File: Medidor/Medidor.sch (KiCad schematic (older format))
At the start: 52 parts, among them J1 TC2030-CTX-TAG_CONECT, SW1 Rotary_Encoder_Switch, SW2 SW_DPST_x2, U1 INA219-INA, U10 spacer, U2 Serial, U3 2450AT18D0100, U4 Fiducial, U5 Fiducial, U6 Fiducial, U7 spacer, U8 spacer, U9 spacer, X1 32MHz

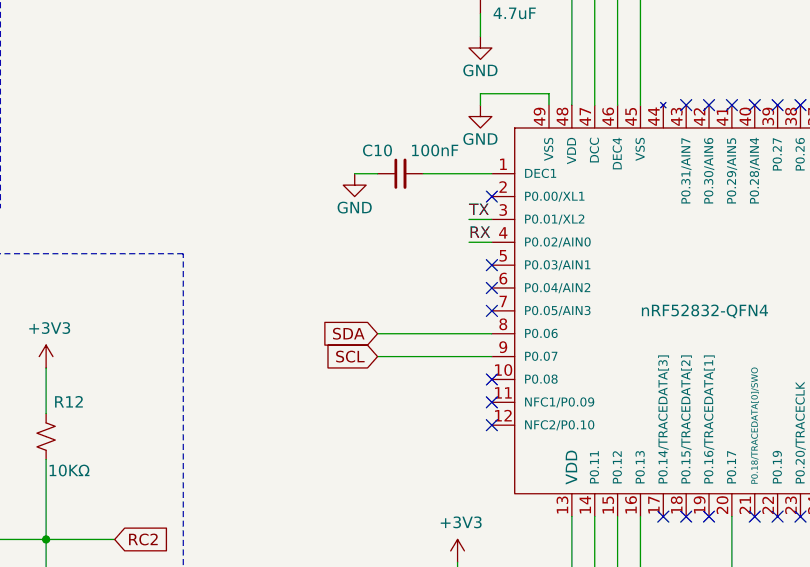
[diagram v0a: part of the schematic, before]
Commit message: Acabamento
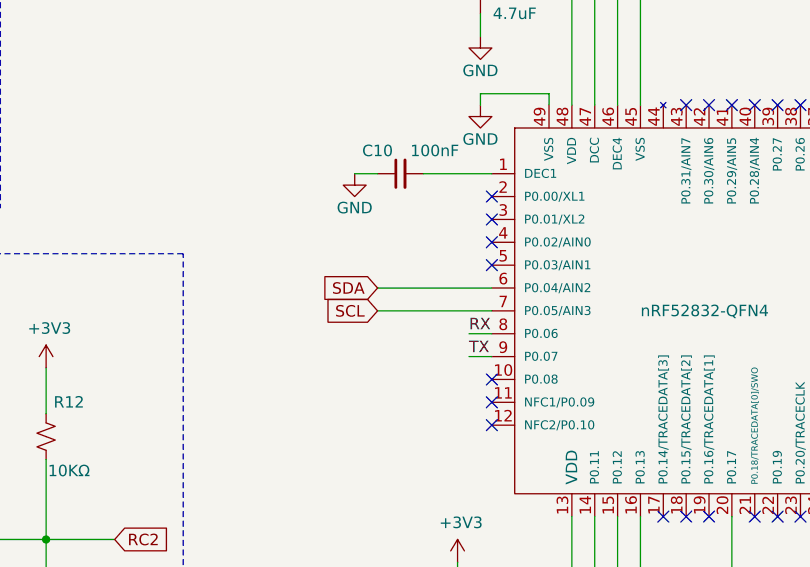
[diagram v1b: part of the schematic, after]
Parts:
- TER1: footprint (none) -> Medidor:Screw
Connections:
- net RX: now also MCU1.8 (P0.06); no longer MCU1.4 (P0.02/AIN0)
- net SCL: now also MCU1.7 (P0.05/AIN3); no longer MCU1.9 (P0.07)
- net SDA: now also MCU1.6 (P0.04/AIN2); no longer MCU1.8 (P0.06)
- net TX: now also MCU1.9 (P0.07); no longer MCU1.3 (P0.01/XL2)
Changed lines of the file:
@@
 Wire Wire Line
 	5400 2500 5400 3550
-Text GLabel 4250 4550 0    50   Input ~ 0
+Text GLabel 4250 4350 0    50   Input ~ 0
 SDA
-Text GLabel 4250 4650 0    50   Input ~ 0
+Text GLabel 4250 4450 0    50   Input ~ 0
 SCL
 NoConn ~ 5800 3550
@@
 LEDMCU
 Wire Wire Line
-	4750 4550 4250 4550
+	4750 4350 4250 4350
 Text GLabel 3700 1950 0    50   Input ~ 0
 LEDMCU
@@
 ALIMENTAÇÂO
 NoConn ~ 4750 3950
-NoConn ~ 4750 4450
 NoConn ~ 4750 4750
 NoConn ~ 4750 4850
-NoConn ~ 4750 4950
 Wire Wire Line
 	1700 7200 1700 6950
@@
 F 0 "TER1" H 10978 1905 50  0000 L CNN
 F 1 "terminal-medidor" H 10978 1860 50  0001 L CNN
-F 2 "" H 10650 2100 50  0001 C CNN
+F 2 "Medidor:Screw" H 10650 2100 50  0001 C CNN
 F 3 "" H 10650 2100 50  0001 C CNN
 	1    10850 1900
@@
 Text Label 4200 6600 0    50   ~ 0
 RX
-Text Label 4650 4050 0    50   ~ 0
+Text Label 4650 4650 0    50   ~ 0
 TX
-Text Label 4650 4150 0    50   ~ 0
+Text Label 4650 4550 0    50   ~ 0
 RX
 Text GLabel 2200 4450 2    50   Input ~ 0
@@
 $EndComp
 Wire Wire Line
-	4250 4650 4750 4650
+	4250 4450 4750 4450
 NoConn ~ 4750 4250
-NoConn ~ 4750 4350
-Wire Wire Line
-	4750 4050 4650 4050
-Wire Wire Line
-	4750 4150 4650 4150
+Wire Wire Line
+	4750 4550 4650 4550
+Wire Wire Line
+	4750 4650 4650 4650
 Wire Wire Line
 	5200 5350 5200 5750
@@
 NoConn ~ 5700 3550
 NoConn ~ 5600 3550
+NoConn ~ 4750 4950
+NoConn ~ 4750 4150
+NoConn ~ 4750 4050
 $EndSCHEMATC

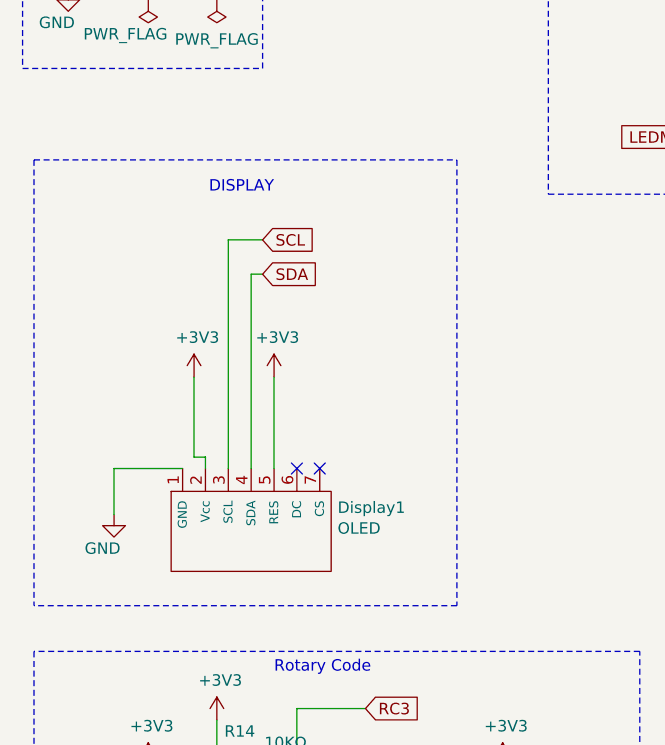
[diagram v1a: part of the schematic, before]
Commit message: corrigindo.
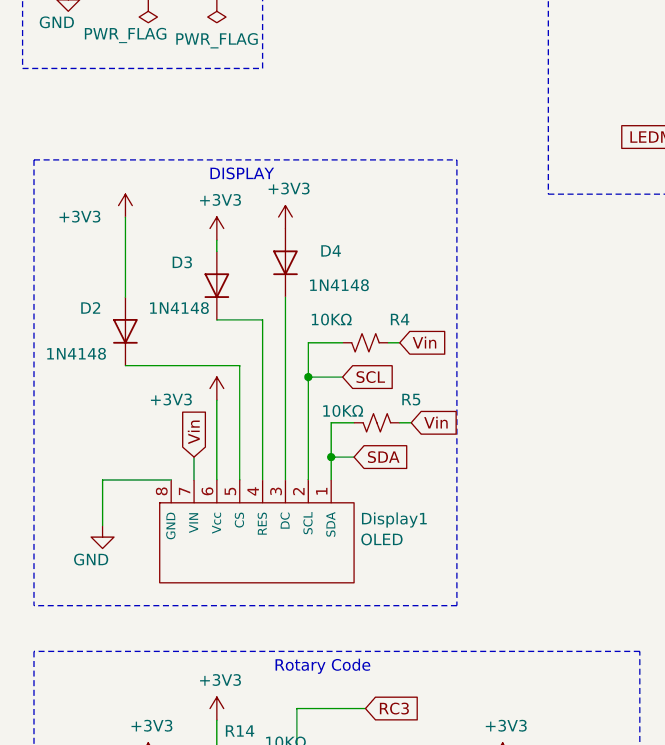
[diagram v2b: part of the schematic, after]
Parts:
- removed Display1: OLED, Medidor:OLED, symbol Medidor-rescue:OLED-medidor
- added D2, D3, D4: 1N4148, Diode_SMD:D_0402_1005Metric, symbol Diode:1N4148
- added Display1: OLED, symbol medidor:OLED
- added R4, R5: 10KΩ, Resistor_SMD:R_0402_1005Metric, symbol Device:R_Small_US
- U1: footprint Medidor:INA219 -> Medidor:INAright
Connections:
- net +3V3: now also D2.2 (A), D3.2 (A), D4.2 (A), Display1.6 (Vcc)
- net GND: now also Display1.8 (GND)
- net SCL: now also Display1.2 (SCL), R4.2
- net SDA: now also Display1.1 (SDA), R5.2
- new net: D4.1 (K), Display1.3 (DC)
- new net: D3.1 (K), Display1.4 (RES)
- new net: D2.1 (K), Display1.5 (CS)
- new net Vin: Display1.7 (VIN), R4.1, R5.1
- no-connect marks 26 -> 24
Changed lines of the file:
@@
 L power:+3V3 #PWR0127
 U 1 1 5D449F7A
-P 1450 3000
-F 0 "#PWR0127" H 1450 2850 50  0001 C CNN
-F 1 "+3V3" H 1465 3173 50  0000 C CNN
-F 2 "" H 1450 3000 50  0001 C CNN
-F 3 "" H 1450 3000 50  0001 C CNN
-	1    1450 3000
-	1    0    0    -1
-$EndComp
-Text GLabel 1750 2400 2    50   Input ~ 0
+P 1150 2300
+F 0 "#PWR0127" H 1150 2150 50  0001 C CNN
+F 1 "+3V3" H 950 2300 50  0000 C CNN
+F 2 "" H 1150 2300 50  0001 C CNN
+F 3 "" H 1150 2300 50  0001 C CNN
+	1    1150 2300
+	1    0    0    -1
+$EndComp
+Text GLabel 2100 3000 2    50   Input ~ 0
 SCL
 Wire Wire Line
-	1750 2400 1600 2400
-Text GLabel 1750 2550 2    50   Input ~ 0
+	2100 3000 1950 3000
+Text GLabel 2150 3350 2    50   Input ~ 0
 SDA
 Wire Wire Line
-	1750 2550 1700 2550
-$Comp
-L power:+3V3 #PWR0128
-U 1 1 5D45DB09
-P 1800 3000
-F 0 "#PWR0128" H 1800 2850 50  0001 C CNN
-F 1 "+3V3" H 1815 3173 50  0000 C CNN
-F 2 "" H 1800 3000 50  0001 C CNN
-F 3 "" H 1800 3000 50  0001 C CNN
-	1    1800 3000
-	1    0    0    -1
-$EndComp
-Text Notes 1800 2200 2    50   ~ 0
+	2150 3350 2050 3350
+Text Notes 1800 2150 2    50   ~ 0
 DISPLAY
 NoConn ~ 6100 5350
@@
 Wire Wire Line
 	7900 4500 7800 4500
-NoConn ~ 1900 3400
-NoConn ~ 2000 3400
-Wire Wire Line
-	1800 3400 1800 3000
-Wire Wire Line
-	1700 2550 1700 3400
-Wire Wire Line
-	1600 2400 1600 3400
-Wire Wire Line
-	1450 3350 1450 3000
-Wire Wire Line
-	1500 3350 1450 3350
-Wire Wire Line
-	1500 3400 1500 3350
-Wire Wire Line
-	1100 3400 1100 3600
-Wire Wire Line
-	1400 3400 1100 3400
+Wire Wire Line
+	2050 3350 2050 3450
+Wire Wire Line
+	1950 3000 1950 3450
+Wire Wire Line
+	1150 2650 1150 2300
+Wire Wire Line
+	1050 3450 1050 3650
+Wire Wire Line
+	1350 3450 1050 3450
 $Comp
 L Device:Rotary_Encoder_Switch SW1
@@
 $EndComp
 $Comp
-L Medidor-rescue:OLED-medidor Display1
-U 1 1 5D5F6826
-P 1700 3700
-F 0 "Display1" H 2078 3829 50  0000 L CNN
-F 1 "OLED" H 2078 3738 50  0000 L CNN
-F 2 "Medidor:OLED" H 1700 3700 50  0001 C CNN
-F 3 "" H 1700 3700 50  0001 C CNN
-	1    1700 3700
-	1    0    0    -1
-$EndComp
-$Comp
 L Medidor-rescue:INA219-INA U1
 U 1 1 5D601474
@@
 F 0 "U1" H 9200 2717 50  0000 C CNN
 F 1 "INA219-INA" H 9200 2626 50  0000 C CNN
-F 2 "Medidor:INA219" H 9200 1850 50  0001 L BNN
+F 2 "Medidor:INAright" H 9200 1850 50  0001 L BNN
 F 3 "" H 9200 1850 50  0001 L BNN
 F 4 "SOT-23-8 Texas Instruments" H 9200 1850 50  0001 L BNN "Campo4"
@@
 L power:GND #PWR0126
 U 1 1 5D406422
-P 1100 3600
-F 0 "#PWR0126" H 1100 3350 50  0001 C CNN
-F 1 "GND" H 1050 3450 50  0000 C CNN
-F 2 "" H 1100 3600 50  0001 C CNN
-F 3 "" H 1100 3600 50  0001 C CNN
-	1    1100 3600
+P 1050 3650
+F 0 "#PWR0126" H 1050 3400 50  0001 C CNN
+F 1 "GND" H 1000 3500 50  0000 C CNN
+F 2 "" H 1050 3650 50  0001 C CNN
+F 3 "" H 1050 3650 50  0001 C CNN
+	1    1050 3650
 	1    0    0    -1
 $EndComp
@@
 NoConn ~ 4750 4150
 NoConn ~ 4750 4050
+$Comp
+L medidor:OLED Display1
+U 1 1 5D82E65F
+P 1650 3750
+F 0 "Display1" H 2178 3879 50  0000 L CNN
+F 1 "OLED" H 2178 3788 50  0000 L CNN
+F 2 "" H 1650 3750 50  0001 C CNN
+F 3 "" H 1650 3750 50  0001 C CNN
+	1    1650 3750
+	1    0    0    -1
+$EndComp
+$Comp
+L Diode:1N4148 D2
+U 1 1 5D8764FA
+P 1150 2800
+F 0 "D2" V 1250 3000 50  0000 R CNN
+F 1 "1N4148" V 1050 3150 50  0000 R CNN
+F 2 "Diode_SMD:D_0402_1005Metric" H 1150 2625 50  0001 C CNN
+F 3 "https://assets.nexperia.com/documents/data-sheet/1N4148_1N4448.pdf" H 1150 2800 50  0001 C CNN
+	1    1150 2800
+	0    -1   -1   0
+$EndComp
+Text GLabel 1450 3350 1    50   Input ~ 0
+Vin
+Wire Wire Line
+	1450 3350 1450 3450
+$Comp
+L power:+3V3 #PWR01
+U 1 1 5D8BB1E1
+P 1550 2400
+F 0 "#PWR01" H 1550 2250 50  0001 C CNN
+F 1 "+3V3" H 1565 2573 50  0000 C CNN
+F 2 "" H 1550 2400 50  0001 C CNN
+F 3 "" H 1550 2400 50  0001 C CNN
+	1    1550 2400
+	1    0    0    -1
+$EndComp
+Wire Wire Line
+	1550 2450 1550 2400
+$Comp
+L Diode:1N4148 D3
+U 1 1 5D8C55EB
+P 1550 2600
+F 0 "D3" V 1650 2800 50  0000 R CNN
+F 1 "1N4148" V 1450 2900 50  0000 R CNN
+F 2 "Diode_SMD:D_0402_1005Metric" H 1550 2425 50  0001 C CNN
+F 3 "https://assets.nexperia.com/documents/data-sheet/1N4148_1N4448.pdf" H 1550 2600 50  0001 C CNN
+	1    1550 2600
+	0    -1   -1   0
+$EndComp
+$Comp
+L power:+3V3 #PWR03
+U 1 1 5D90BE04
+P 1850 2350
+F 0 "#PWR03" H 1850 2200 50  0001 C CNN
+F 1 "+3V3" H 1865 2523 50  0000 C CNN
+F 2 "" H 1850 2350 50  0001 C CNN
+F 3 "" H 1850 2350 50  0001 C CNN
+	1    1850 2350
+	1    0    0    -1
+$EndComp
+$Comp
+L Diode:1N4148 D4
+U 1 1 5D90BE0B
+P 1850 2500
+F 0 "D4" V 1900 2350 50  0000 R CNN
+F 1 "1N4148" V 1750 2400 50  0000 R CNN
+F 2 "Diode_SMD:D_0402_1005Metric" H 1850 2325 50  0001 C CNN
+F 3 "https://assets.nexperia.com/documents/data-sheet/1N4148_1N4448.pdf" H 1850 2500 50  0001 C CNN
+	1    1850 2500
+	0    -1   -1   0
+$EndComp
+Wire Wire Line
+	1850 2650 1850 3450
+Wire Wire Line
+	1550 2750 1750 2750
+Wire Wire Line
+	1750 2750 1750 3450
+Wire Wire Line
+	1150 2950 1650 2950
+Wire Wire Line
+	1650 2950 1650 3450
+$Comp
+L power:+3V3 #PWR02
+U 1 1 5D96BC9C
+P 1550 3100
+F 0 "#PWR02" H 1550 2950 50  0001 C CNN
+F 1 "+3V3" H 1350 3100 50  0000 C CNN
+F 2 "" H 1550 3100 50  0001 C CNN
+F 3 "" H 1550 3100 50  0001 C CNN
+	1    1550 3100
+	1    0    0    -1
+$EndComp
+Wire Wire Line
+	1550 3450 1550 3100
+$Comp
+L Device:R_Small_US R4
+U 1 1 5D977F12
+P 2200 2850
+F 0 "R4" V 2300 3000 50  0000 C CNN
+F 1 "10KΩ" V 2300 2700 50  0000 C CNN
+F 2 "Resistor_SMD:R_0402_1005Metric" H 2200 2850 50  0001 C CNN
+F 3 "~" H 2200 2850 50  0001 C CNN
+	1    2200 2850
+	0    1    -1   0
+$EndComp
+Wire Wire Line
+	2100 2850 1950 2850
+Wire Wire Line
+	1950 2850 1950 3000
+Connection ~ 1950 3000
+Text GLabel 2350 2850 2    50   Input ~ 0
+Vin
+Wire Wire Line
+	2300 2850 2350 2850
+$Comp
+L Device:R_Small_US R5
+U 1 1 5D9FCC2B
+P 2250 3200
+F 0 "R5" V 2350 3350 50  0000 C CNN
+F 1 "10KΩ" V 2300 3050 50  0000 C CNN
+F 2 "Resistor_SMD:R_0402_1005Metric" H 2250 3200 50  0001 C CNN
+F 3 "~" H 2250 3200 50  0001 C CNN
+	1    2250 3200
+	0    1    -1   0
+$EndComp
+Text GLabel 2400 3200 2    50   Input ~ 0
+Vin
+Wire Wire Line
+	2400 3200 2350 3200
+Wire Wire Line
+	2150 3200 2050 3200
+Wire Wire Line
+	2050 3200 2050 3350
+Connection ~ 2050 3350
 $EndSCHEMATC
